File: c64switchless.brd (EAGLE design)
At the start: 22.8 x 44.1 mm, 12 parts, among them IC1 27C256, IC2 PIC12F629P, X1 B4B-ZR

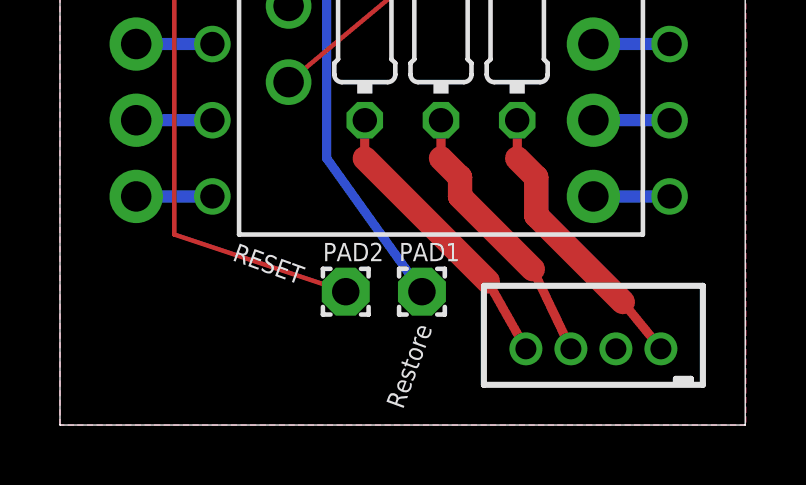
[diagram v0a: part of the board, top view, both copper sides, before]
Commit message: Revision + silkscreen text
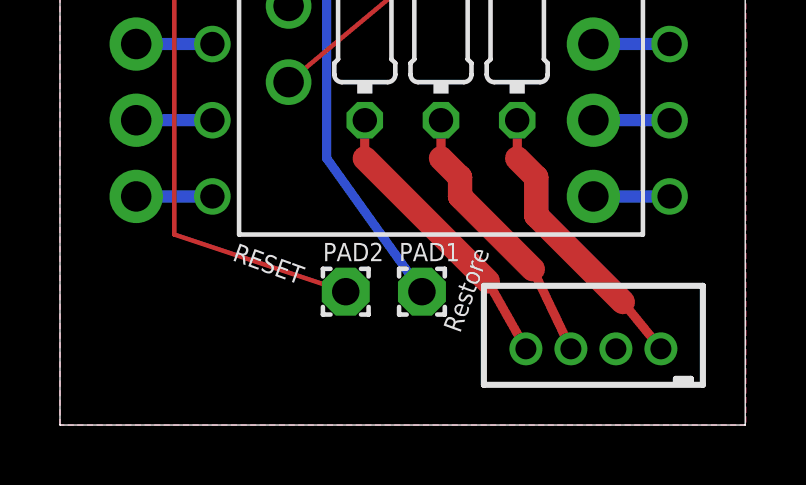
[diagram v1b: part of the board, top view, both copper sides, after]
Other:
- board text added: "B"
- board text added: "G"
- board text added: "Gnd"
- board text added: "LED"
- board text added: "R"
- board text added: "Revision 1"
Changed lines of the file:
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@@
 <setting verticaltext="up"/>
 </settings>
-<grid distance="0.05" unitdist="inch" unit="mm" style="lines" multiple="1" display="yes" altdistance="0.025" altunitdist="inch" altunit="inch"/>
+<grid distance="0.05" unitdist="inch" unit="inch" style="lines" multiple="1" display="yes" altdistance="0.025" altunitdist="inch" altunit="inch"/>
 <layers>
 <layer number="1" name="Top" color="4" fill="1" visible="yes" active="yes"/>
@@
 <text x="1.27" y="1.27" size="0.6096" layer="29" font="fixed">Quad Kernal Switch</text>
 <text x="5.715" y="5.5" size="0.6096" layer="21" rot="R340">RESET</text>
-<text x="11.43" y="0.5" size="0.6096" layer="21" rot="R70">Restore</text>
+<text x="13.335" y="3.04" size="0.6096" layer="21" rot="R70">Restore</text>
+<text x="13.97" y="1.27" size="0.6096" layer="23" font="fixed" rot="R90">LED</text>
+<text x="3.175" y="0.635" size="0.6096" layer="23" font="fixed">Revision 1</text>
+<text x="19.812" y="0.635" size="0.6096" layer="23" font="fixed">R</text>
+<text x="16.764" y="0.635" size="0.6096" layer="23" font="fixed">G</text>
+<text x="15.24" y="0.635" size="0.6096" layer="23" font="fixed">B</text>
+<text x="17.78" y="0.635" size="0.6096" layer="23" font="fixed">Gnd</text>
 </plain>
 <attributes>
